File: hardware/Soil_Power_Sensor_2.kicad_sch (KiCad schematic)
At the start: 4 parts, among them J1 Conn_01x02, SW3 SW_SPDT

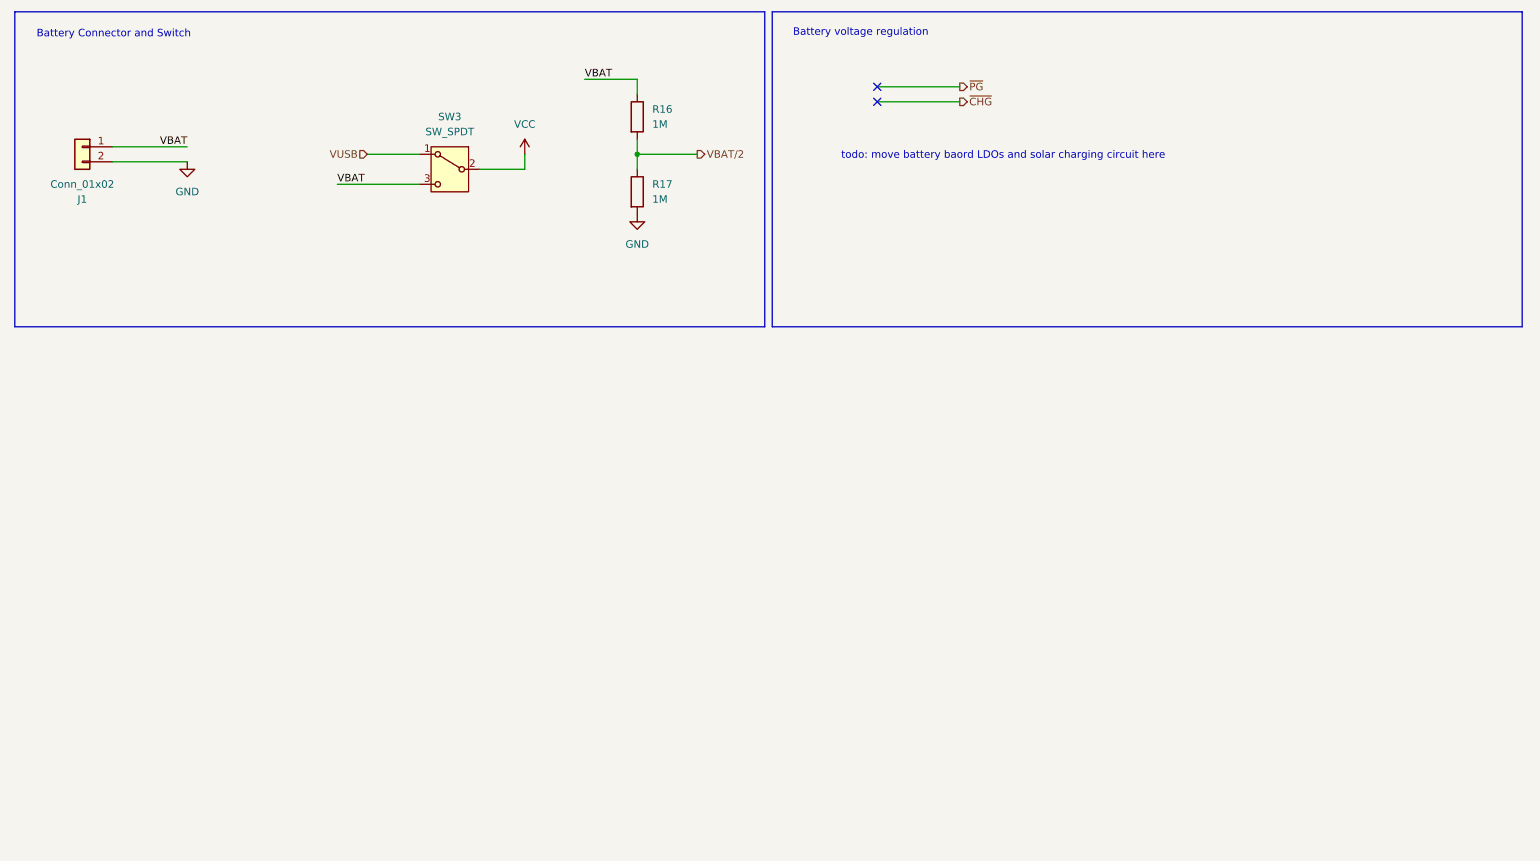
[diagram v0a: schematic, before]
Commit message: usb ttl components
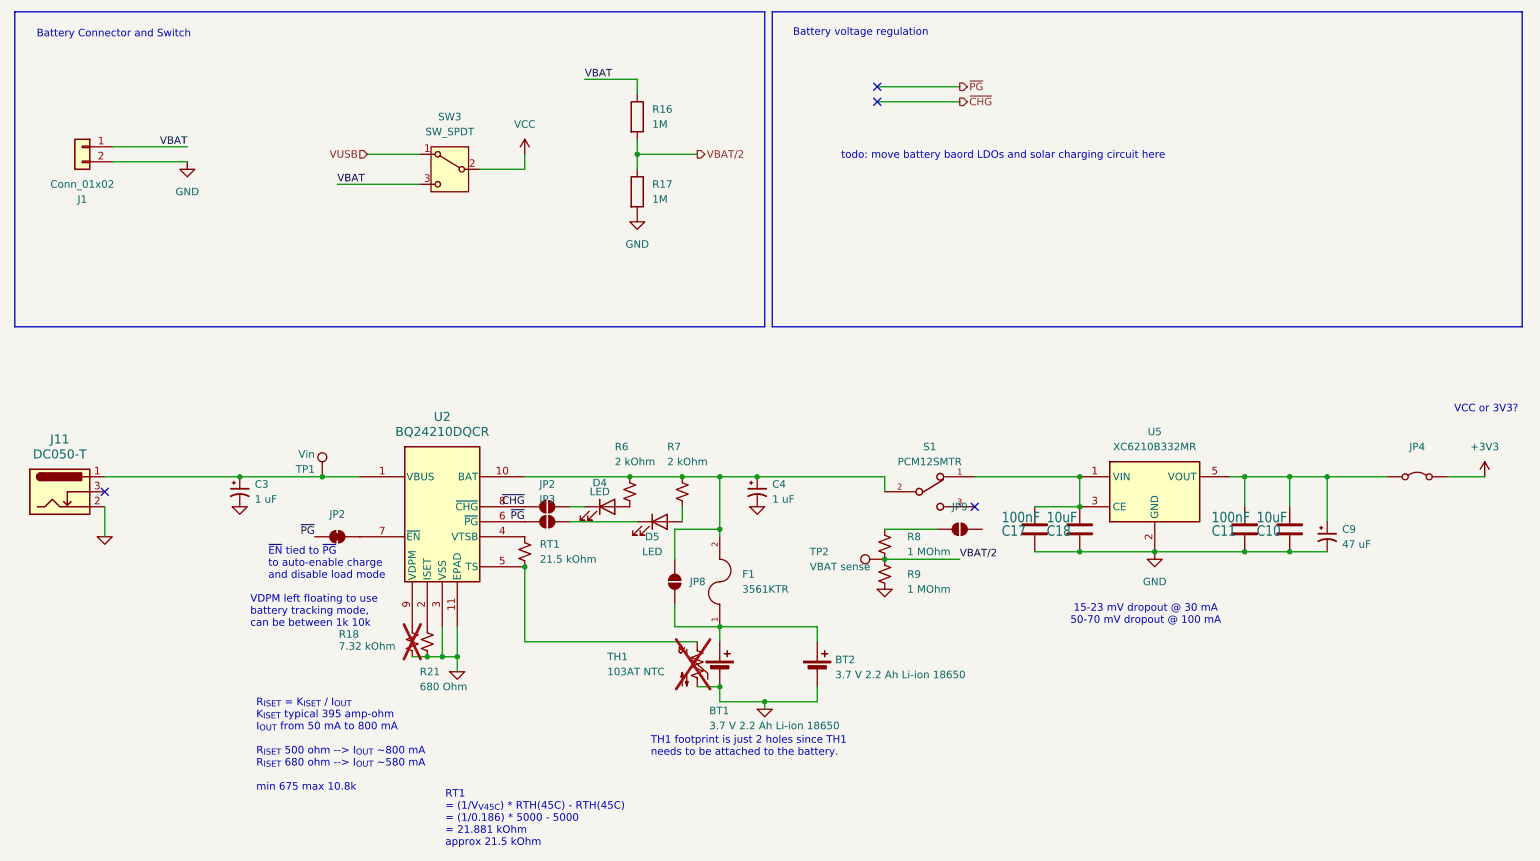
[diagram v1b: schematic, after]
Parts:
- added BT1, BT2: 3.7 V 2.2 Ah Li-ion 18650, footprints:MY-18650-02, symbol Device:Battery_Cell
- added C10, C18: 10uF, Capacitor_SMD:C_0603_1608Metric, symbol Device:C
- added C11, C17: 100nF, Capacitor_SMD:C_0603_1608Metric, symbol Device:C
- added C3, C4: 1 uF, Capacitor_SMD:C_0603_1608Metric, symbol Device:C_Polarized_Small_US
- added C9: 47 uF, Capacitor_SMD:C_0603_1608Metric, symbol Device:C_Polarized_Small_US
- added D4, D5: LED, LED_SMD:LED_0603_1608Metric, symbol Device:LED
- added F1: 3561KTR, 3561KTR:FUSE_3561KTR, symbol 3561KTR:3561KTR
- added J11: DC050-T, DC050-T:DC050-T, symbol Connector:Barrel_Jack_Switch
- added JP2: SolderJumper_2_Bridged, Jumper:SolderJumper-2_P1.3mm_Bridged_RoundedPad1.0x1.5mm, symbol Jumper:SolderJumper_2_Bridged
- added JP2, JP3, JP8, JP9: SolderJumper_2_Open, Jumper:SolderJumper-2_P1.3mm_Open_RoundedPad1.0x1.5mm, symbol Jumper:SolderJumper_2_Open
- added JP4: Jumper_2_Bridged, symbol Jumper:Jumper_2_Bridged
- added R18: 7.32 kOhm, Resistor_SMD:R_0603_1608Metric, symbol Device:R_Small_US
- added R21: 680 Ohm, Resistor_SMD:R_0603_1608Metric, symbol Device:R_Small_US
- added R6, R7: 2 kOhm, Resistor_SMD:R_0603_1608Metric, symbol Device:R_Small_US
- added R8, R9: 1 MOhm, Resistor_SMD:R_0603_1608Metric, symbol Device:R_Small_US
- added RT1: 21.5 kOhm, Resistor_SMD:R_0603_1608Metric, symbol Device:R_Small_US
- added S1: PCM12SMTR, Button_Switch_SMD:SW_SPDT_PCM12, symbol JS102011SAQN:JS102011SAQN
- added TH1: 103AT NTC, Connector_PinHeader_2.54mm:PinHeader_1x02_P2.54mm_Vertical, symbol Device:Thermistor_NTC_US
- added TP1: Vin, TestPoint:TestPoint_Pad_D1.5mm, symbol Connector:TestPoint
- added TP2: VBAT sense, TestPoint:TestPoint_Pad_D1.5mm, symbol Connector:TestPoint
- added U2: BQ24210DQCR, BQ24210:DQC10_P84X2P4, symbol BQ24210:BQ24210DQCR
- added U5: XC6210B332MR, Package_TO_SOT_SMD:SOT-23-5, symbol Regulator_Linear:XC6210B332MR
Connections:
- net GND: now also C10.2, C11.2, C17.2, C18.2, C9.2, U5.2 (GND)
- net VBAT/2: now also R8.2, R9.1, TP2.1
- net ~{CHG}: now also JP2.1 (A), U2.8 (~{CHG})
- net ~{PG}: now also JP2.1 (A), JP3.1 (A), U2.6 (~{PG})
- new net: C4.1, F1.2, JP8.2 (B), R6.1, R7.1, S1.2, U2.10 (BAT)
- new net: C17.1, C18.1, S1.1, U5.1 (VIN), U5.3 (CE)
- new net: C10.1, C11.1, C9.1, JP4.1 (A), U5.5 (VOUT)
- new net: D4.1 (K), JP2.2 (B)
- new net: D4.2 (A), R6.2
- new net: RT1.1, U2.4 (VTSB)
- new net: RT1.2, TH1.1, U2.5 (TS)
- new net: JP2.2 (B), U2.7 (~{EN})
- new net: C3.1, J11.1, TP1.1, U2.1 (VBUS)
- new net: BT1.1 (+), BT2.1 (+), F1.1, JP8.1 (A)
- new net: D5.1 (K), JP3.2 (B)
- new net: D5.2 (A), R7.2
- new net: JP9.1 (A), R8.1
- new net: R18.1, U2.9 (VDPM)
- new net: R21.1, U2.2 (ISET)
- new net +3V3: JP4.2 (B)
- new net 0: BT1.2 (-), BT2.2 (-), C3.2, C4.2, J11.2, R18.2, R21.2, R9.2, TH1.2, U2.11 (EPAD), U2.3 (VSS)
- no-connect marks 2 -> 4
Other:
- note added: "15-23 mV dropout @ 30 mA 50-70 mV dropout @ 100 mA"
- note added: "RT1 = (1/V_{V45C}) * RTH(45C) - RTH(45C) = (1/0.186) * 5000 - 5000 = 21.881 kOhm approx 21.5 kOhm"
- note added: "R_{ISET} = K_{ISET} / I_{OUT} K_{ISET} typical 395 amp-ohm I_{OUT} from 50 mA to 800 mA R_{ISET} 500 ohm --> I_{OUT} ~800 mA R_{ISET} 680 ohm --> I_{OUT} ~580 mA min 675 max 10.8k"
- note added: "TH1 footprint is just 2 holes since TH1 needs to be attached to the battery."
- note added: "VCC or 3V3?"
- note added: "VDPM left floating to use battery tracking mode, can be between 1k 10k"
- note added: "~{EN} tied to ~{PG} to auto-enable charge and disable load mode"
